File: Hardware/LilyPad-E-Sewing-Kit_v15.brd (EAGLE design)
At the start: 50.9 x 52.1 mm, 53 parts

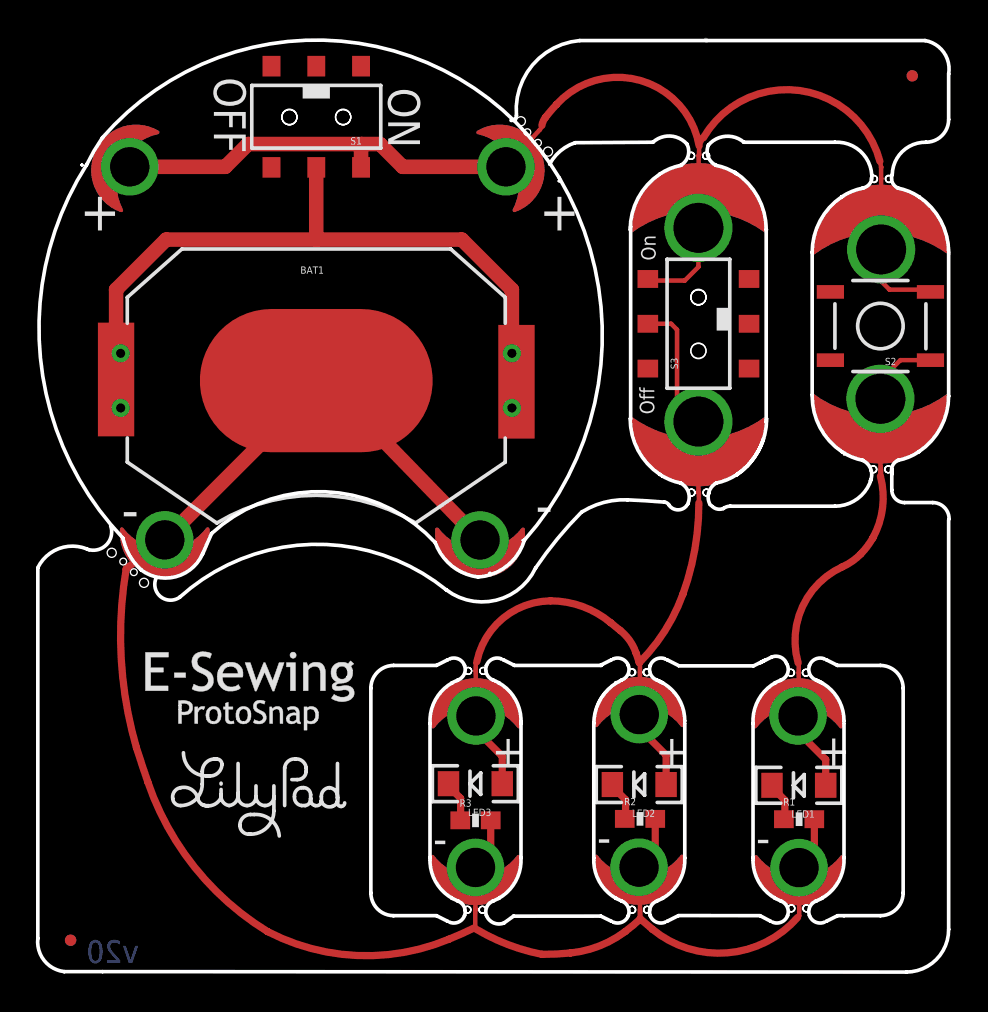
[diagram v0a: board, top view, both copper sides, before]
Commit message: Put it back on grid....
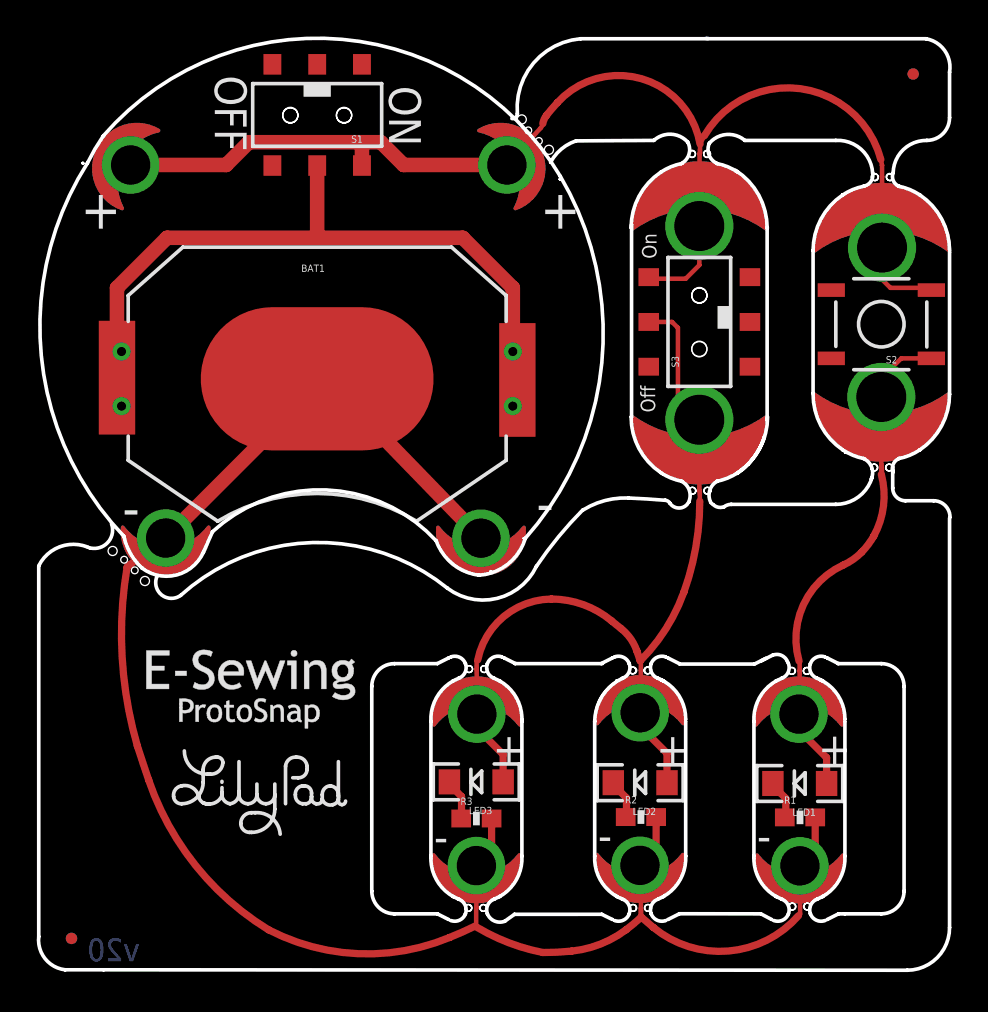
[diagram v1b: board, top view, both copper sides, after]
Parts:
- moved S3 0.11 mm to (36.9, 36.2)
- moved SLIDEON 0.11 mm to (36.9, 41.3)
- moved LED+2 0.11 mm to (33.6, 14.4)
- moved LED1 0.11 mm to (42.5, 10.4)
- moved LED2 0.11 mm to (33.6, 10.4)
- moved R2 0.11 mm to (33.6, 8.53)
- moved MB6 0.11 mm to (24.4, 3.45)
- moved MB8 0.11 mm to (42.5, 3.53)
- moved BATB- 0.11 mm to (7.09, 24.1)
- moved MB- 0.11 mm to (5.05, 22.6)
- moved LED-1 0.11 mm to (42.5, 5.80)
- moved LED3 0.11 mm to (24.4, 10.5)
- moved BATB-2 0.11 mm to (24.7, 24.1)
- moved LED+3 0.11 mm to (24.5, 14.3)
- moved MB5 0.11 mm to (24.4, 16.8)
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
